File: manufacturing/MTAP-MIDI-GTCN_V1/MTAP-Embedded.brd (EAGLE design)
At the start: 30.5 x 45.1 mm, 32 parts, among them IC1 ESP32-WROOM-32UE-N8, IC2 AMS1117-3.3, J1 629105150521

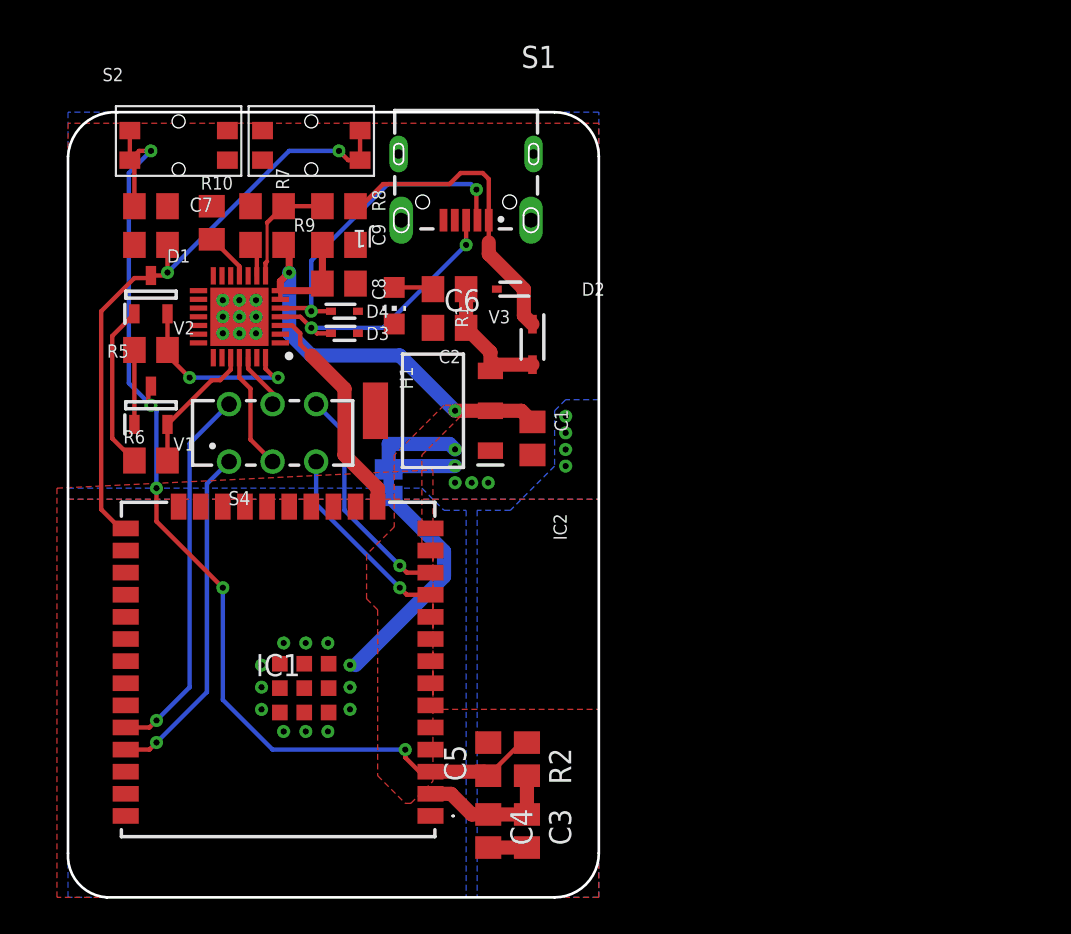
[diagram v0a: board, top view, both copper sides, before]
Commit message: adp adc #3 pcb
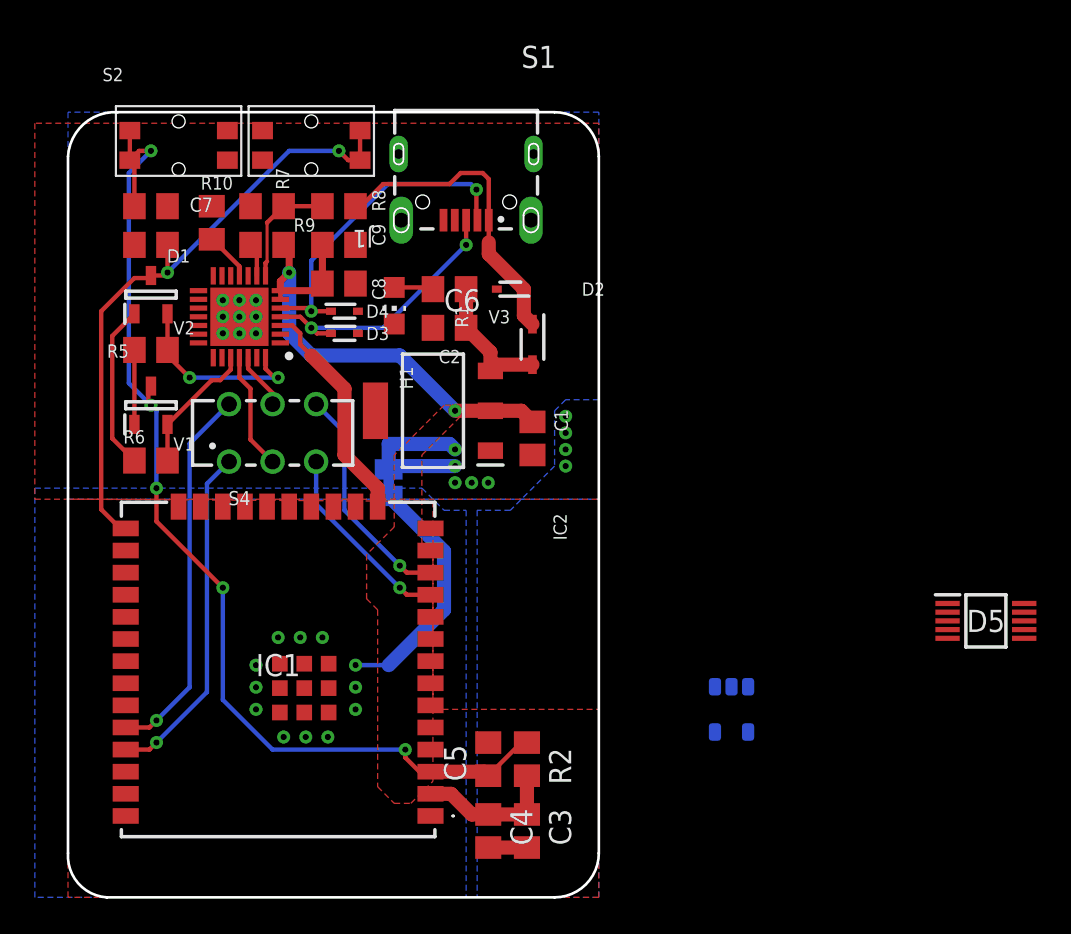
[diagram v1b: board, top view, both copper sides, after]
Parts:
- added D5: MCP33131-05-E, adc-dac_GruS:MSOP10
- added N1: TC2015, vreg_GruS:SOT-23-5
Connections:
- new net +1V8: D5.2, N1.5
- new net ADI: D5.9
- new net AGND: D5.4, D5.5, N1.4
- new net N$10: N1.2
- new net N$11: D5.3
- new net N$6: D5.7
- new net N$7: D5.8
- new net N$8: N1.3
- new net N$9: D5.1
- net +3V3: now also N1.1
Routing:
- net GND: track 29.0 -> 29.8 mm
